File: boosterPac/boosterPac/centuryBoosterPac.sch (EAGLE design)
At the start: 37 parts, among them IC1 317T, J1 22-05-7028-02, J2 22-05-7028-02, Q1 BSS123

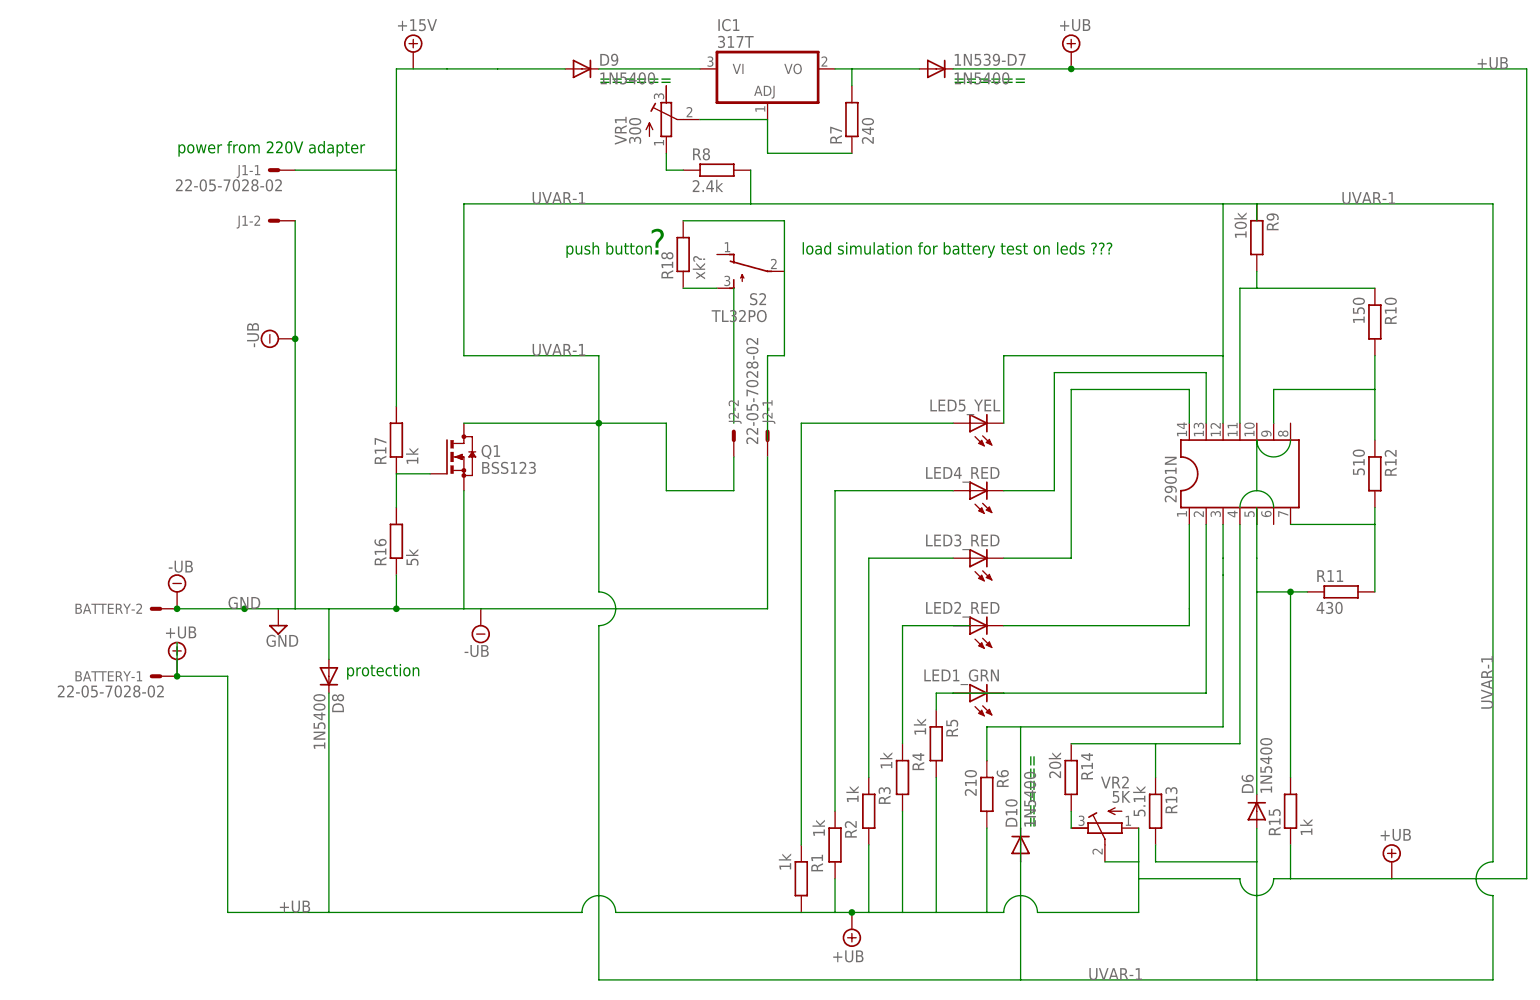
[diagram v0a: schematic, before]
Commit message: reg save
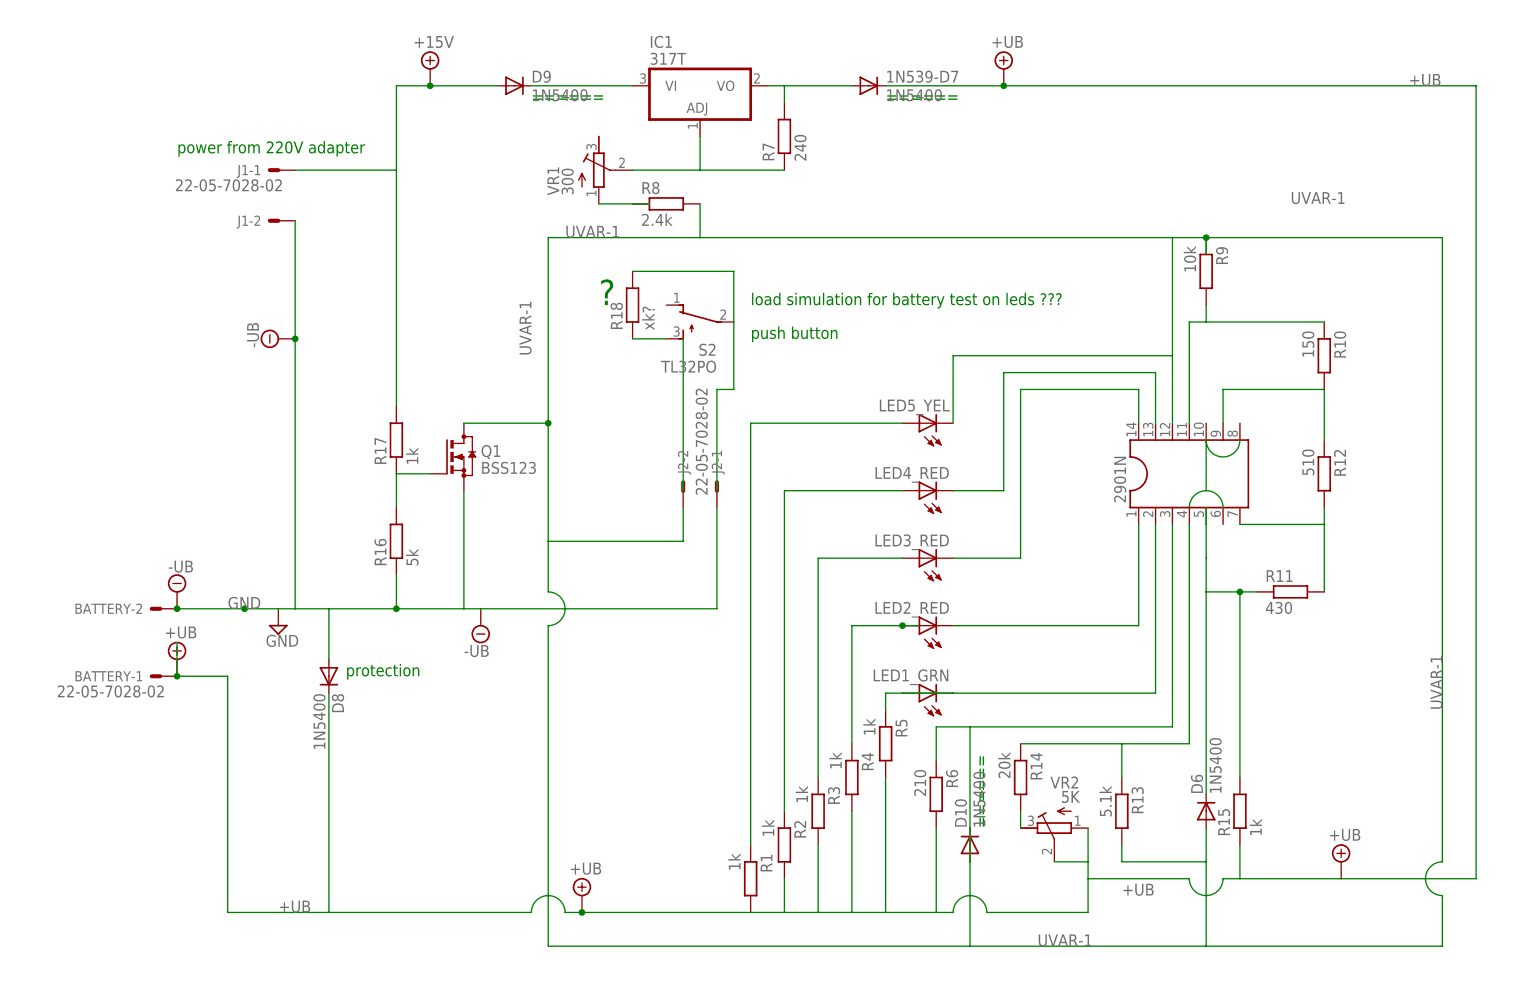
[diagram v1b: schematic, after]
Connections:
- net N$15: now also LED2_RED.A
- net N$3: no longer R8.1
- net UVAR-1: now also R9.1
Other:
- moved on the sheet: 1N539-D7, 2901N, D10, D6, D9, IC1, J2-1, J2-2, LED1_GRN, LED2_RED, LED3_RED, LED4_RED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
